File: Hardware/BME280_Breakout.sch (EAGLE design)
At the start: 19 parts, among them U1 BME280

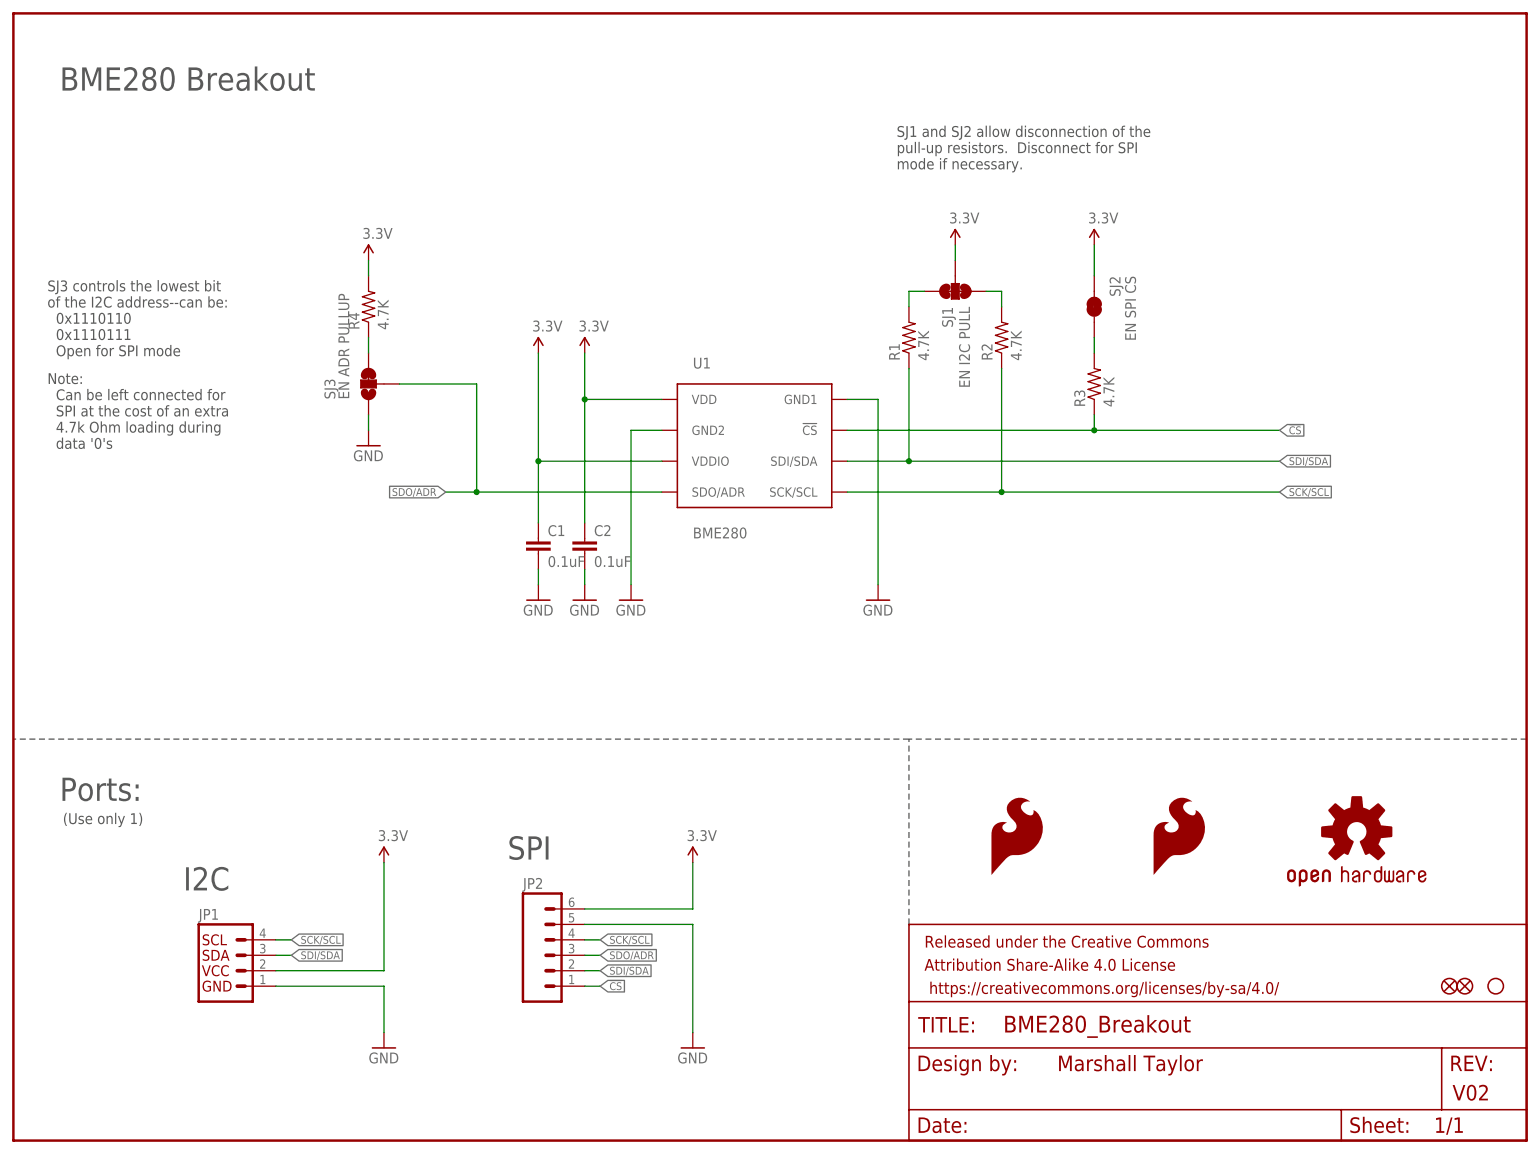
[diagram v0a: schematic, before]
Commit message: Ready for review
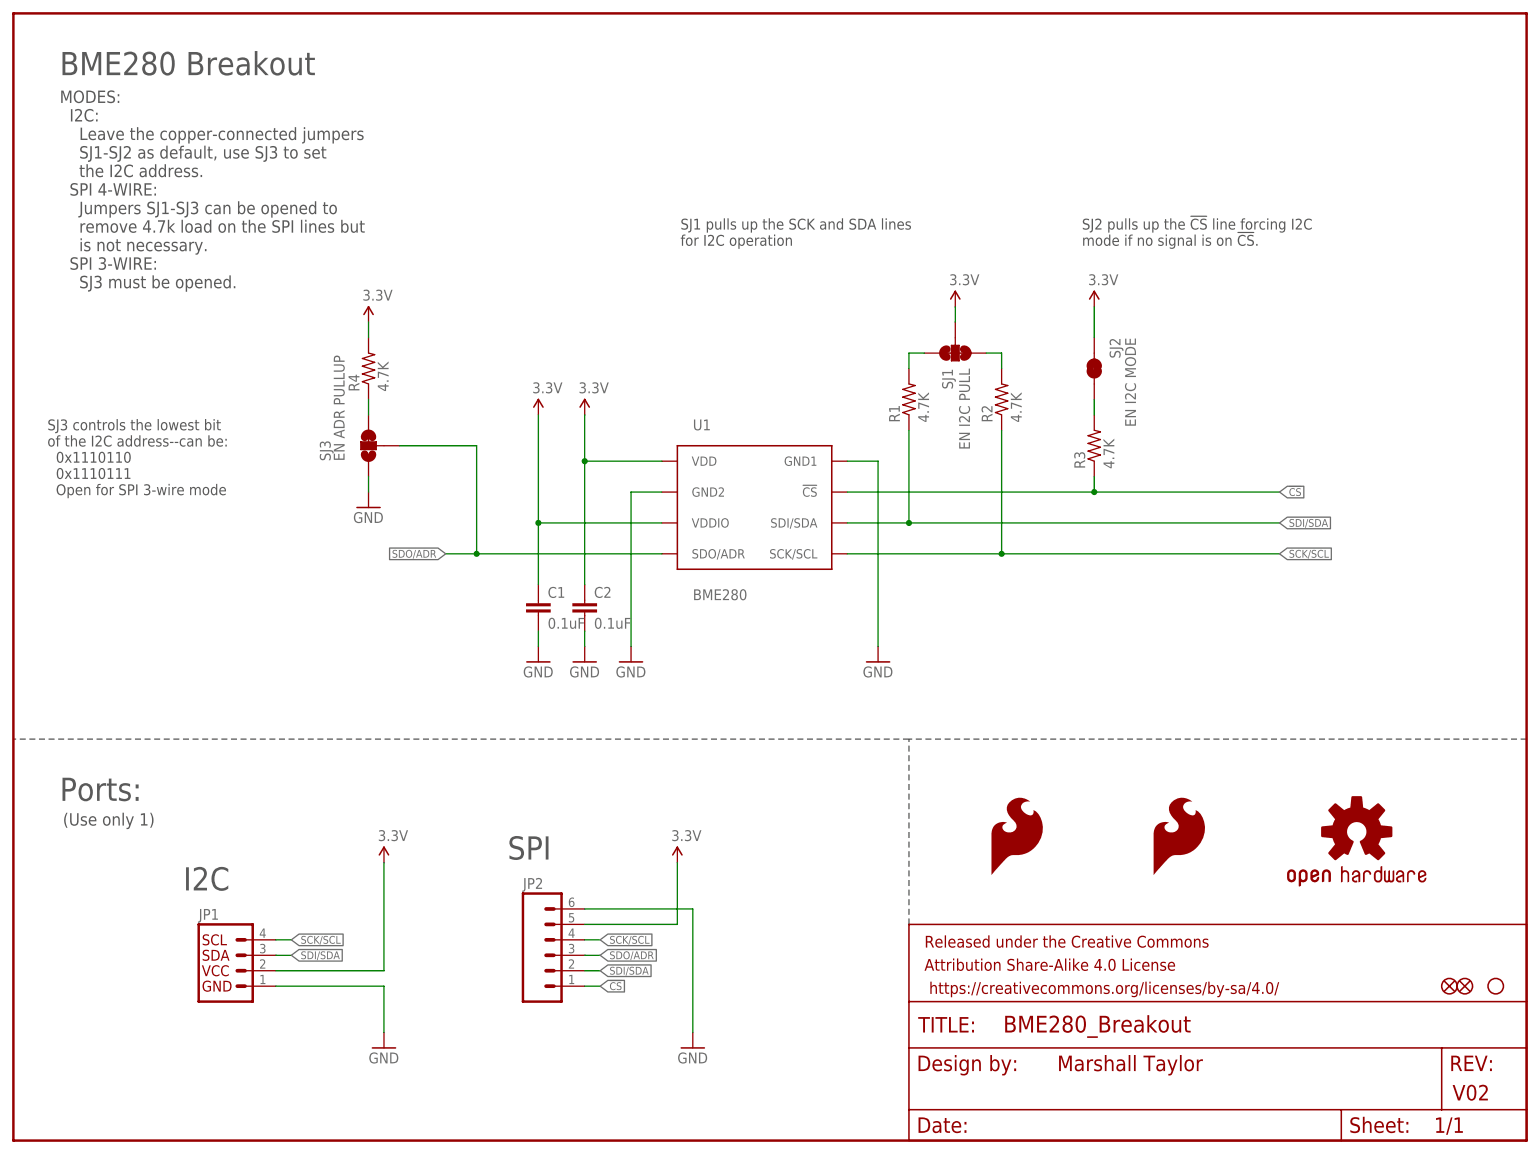
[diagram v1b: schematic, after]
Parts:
- SJ2: value EN SPI CS -> EN I2C MODE
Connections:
- net 3.3V: now also JP2.5; no longer JP2.6
- net GND: now also JP2.6; no longer JP2.5
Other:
- note added: "MODES: I2C: Leave the copper-connected jumpers SJ1-SJ2 as default, use SJ3 to set the I2C address. SPI 4-WIRE: Jumpers SJ1-SJ3 can be opened to remove 4.7k load on the SPI lines but is not necessary. SPI 3-WIRE: SJ3 must be opened."
- note added: "SJ1 pulls up the SCK and SDA lines for I2C operation"
- note added: "SJ2 pulls up the !CS! line forcing I2C mode if no signal is on !CS!."
- note added: "SJ3 controls the lowest bit of the I2C address--can be: 0x1110110 0x1110111 Open for SPI 3-wire mode"
- note removed: "Note: Can be left connected for SPI at the cost of an extra 4.7k Ohm loading during data '0's"
- note removed: "SJ1 and SJ2 allow disconnection of the pull-up resistors. Disconnect for SPI mode if necessary."
- note removed: "SJ3 controls the lowest bit of the I2C address--can be: 0x1110110 0x1110111 Open for SPI mode"
- moved on the sheet: C1, C2, R1, R2, R3, R4, SJ1, SJ2, SJ3, U1
